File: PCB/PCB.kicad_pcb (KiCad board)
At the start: 2 copper layers, 53.3 x 73.7 mm, 23 parts, among them J1 PWR,A0, J10 D8-D10, J11 D0-D7, J12 GrowLight Out, J2 12V, J3 LightSensor, J4 Pump1, J5 Sensor1, J6 GrowLight In, J7 Pump2, J8 Sensor2, J9 Setup, K1 Relay1, K2 RelayGrowlight, K3 Relay2, Q1 BC337, Q2 BC337, Q3 BC337, U1 AM2302, U2 74HC4051

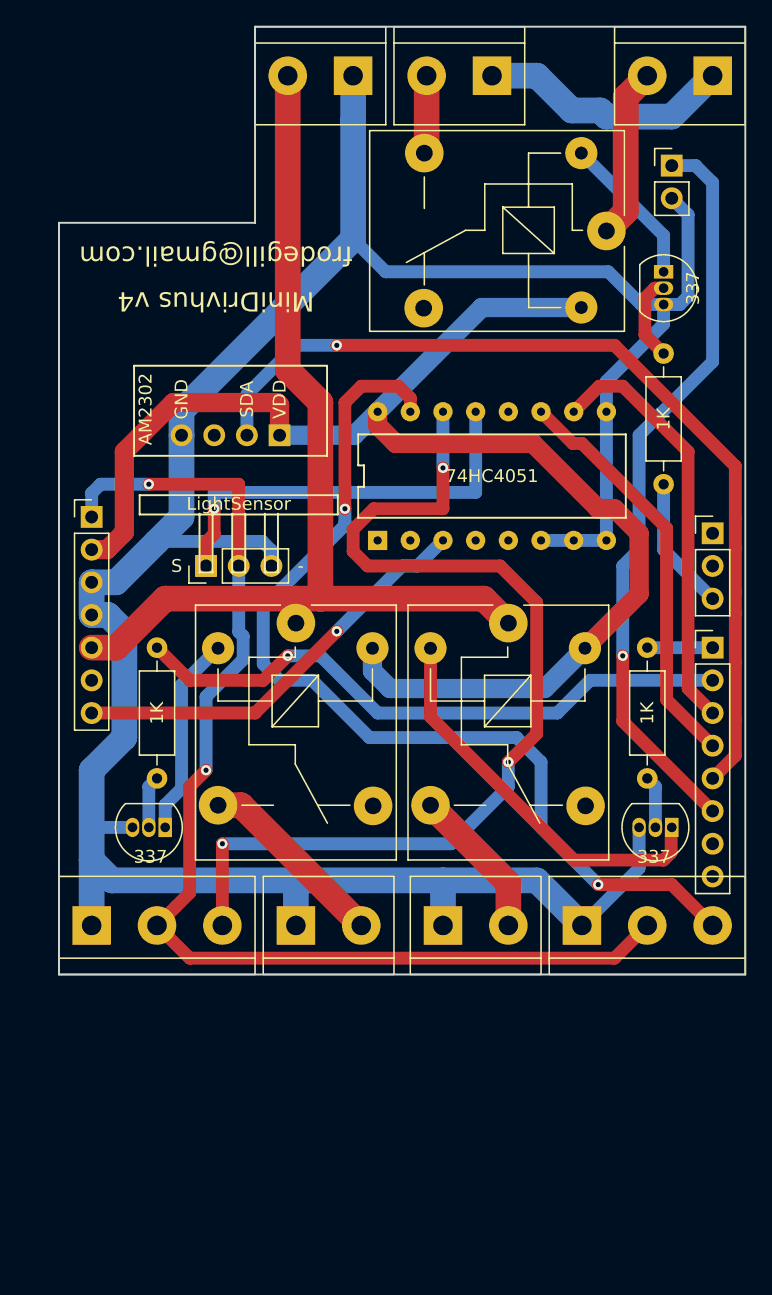
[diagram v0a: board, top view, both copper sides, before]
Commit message: Kicad-files for MivinDrivhus_v5
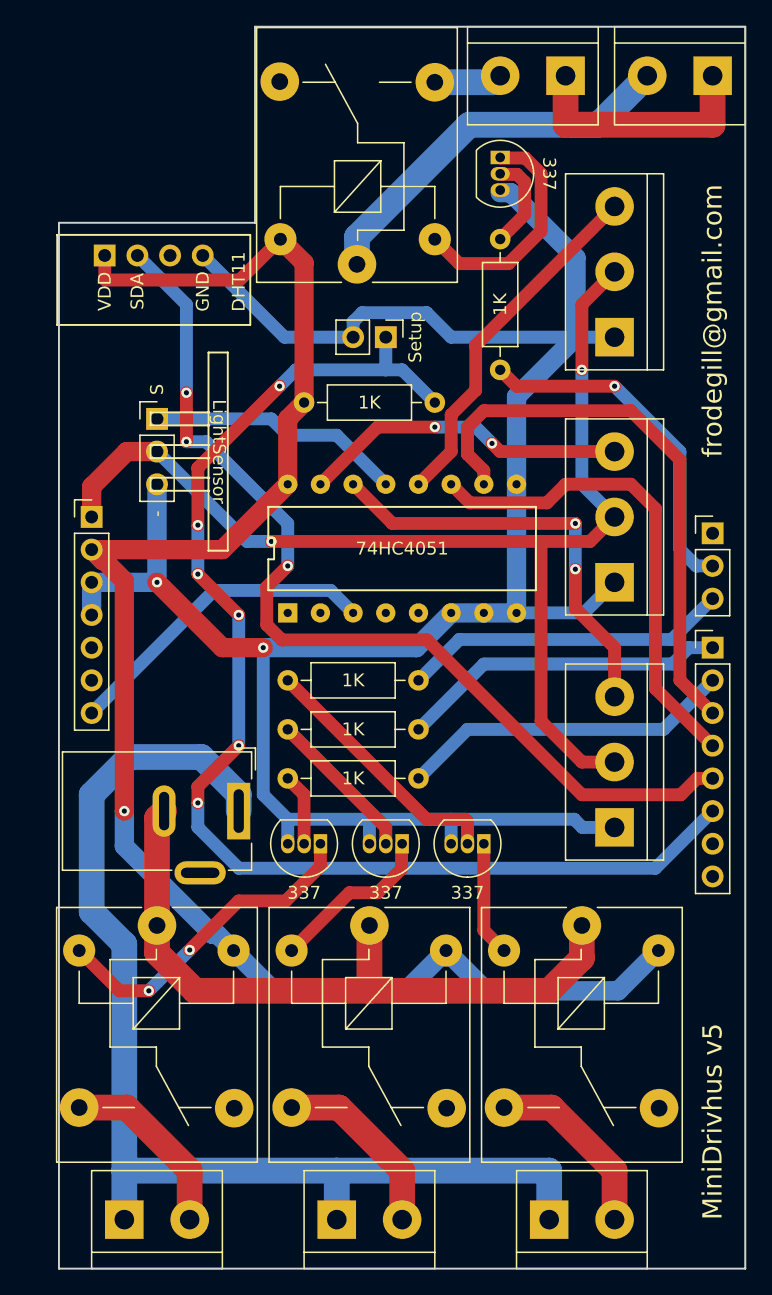
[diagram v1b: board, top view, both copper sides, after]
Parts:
- added J13: Pump3, TerminalBlock:TerminalBlock_bornier-2_P5.08mm, F.Cu at (177.8, 128.3)
- added J14: Sensor3, TerminalBlock:TerminalBlock_bornier-3_P5.08mm, F.Cu at (182.9, 59.7)
- added K4: Relay3, Relay_THT:Relay_SPDT_SANYOU_SRD_Series_Form_C, F.Cu at (180.3, 105.4)
- added Q4: BC337, Package_TO_SOT_THT:TO-92_Inline, F.Cu at (172.7, 99.1)
- added R4: 1K, Resistor_THT:R_Axial_DIN0207_L6.3mm_D2.5mm_P10.16mm_Horizontal, F.Cu at (158.8, 64.8)
- added R5: 1K, Resistor_THT:R_Axial_DIN0207_L6.3mm_D2.5mm_P10.16mm_Horizontal, F.Cu at (157.5, 86.4)
- J2: value 12V -> Pump In; footprint TerminalBlock:TerminalBlock_bornier-2_P5.08mm -> Connector_BarrelJack:BarrelJack_Wuerth_6941xx301002
- U1: value AM2302 -> DHT11
- moved J2 57.8 mm to (153.7, 96.5), turned to 270 degrees
- moved J5 41.3 mm to (182.9, 97.8), turned to 90 degrees
- moved R3 28.2 mm to (157.5, 90.2), turned to 0 degrees
- moved J8 26.8 mm to (182.9, 78.7), turned to 90 degrees
- moved J4 26.5 mm to (144.8, 128.3)
- moved J9 25.9 mm to (165.1, 59.7), turned to 270 degrees
- moved K1 25.9 mm to (147.3, 105.4)
- moved K3 25.9 mm to (163.8, 105.4)
- moved J7 24.3 mm to (161.3, 128.3)
- moved Q3 21.0 mm to (166.4, 99.1)
- moved K2 19.6 mm to (162.9, 54.0), turned to 90 degrees
- moved Q2 15.5 mm to (174.0, 45.7)
- moved R2 15.5 mm to (174.0, 52.1)
- moved U1 15.2 mm to (147.1, 53.3), turned to 0 degrees
- moved Q1 12.1 mm to (160.0, 99.1)
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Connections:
- J1 pad 5: +12V -> (no net)
- J10 pad 2: (no net) -> Net-(J10-Pad2)
- J2 pad 1: GND -> Net-(J13-Pad1)
- J2 pad 2: +12V -> Net-(J2-Pad2)
- J4 pad 1: GND -> Net-(J13-Pad1)
- J7 pad 1: GND -> Net-(J13-Pad1)
- K1 pad 1: +12V -> Net-(J2-Pad2)
- K3 pad 1: +12V -> Net-(J2-Pad2)
- R2 pad 2: Net-(J10-Pad3) -> Net-(J10-Pad2)
- U2 pad 12: (no net) -> Net-(J14-Pad3)
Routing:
- net Net-(J13-Pad1): track 0.00 -> 89.9 mm
- net +12V: track 78.3 -> 0.00 mm
- net Net-(J2-Pad2): track 0.00 -> 54.2 mm
- net Net-(J8-Pad3): track 76.3 -> 25.5 mm
- net Net-(J5-Pad3): track 78.4 -> 33.3 mm, vias 3 -> 2
- net Net-(J11-Pad6): track 58.4 -> 98.9 mm, vias 1 -> 6
- net GND: track 210.4 -> 174.9 mm, vias 0 -> 2
- net Net-(J14-Pad3): track 0.00 -> 27.9 mm
- net Net-(J10-Pad2): track 0.00 -> 27.3 mm, vias 0 -> 1
- net Net-(J11-Pad2): track 47.9 -> 26.0 mm, vias 1 -> 0
- net Net-(J11-Pad1): track 5.08 -> 25.5 mm
- net Net-(Q4-Pad2): track 0.00 -> 20.3 mm
- net +5V: track 108.7 -> 128.7 mm, vias 0 -> 1
- net Net-(K3-Pad2): track 30.9 -> 13.1 mm
- net Net-(J12-Pad2): track 13.4 -> 29.9 mm
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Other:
- board size 53.3 x 73.7 mm -> 53.3 x 96.5 mm
- board text added: "- +"
- board text added: "MiniDrivhus v5"
- board text added: "Pump3"
- board text added: "Sensor3"
- board text removed: "12V"
- board text removed: "3V 5V GND GND 12V A0"
- board text removed: "D10 D9 D8"
- board text removed: "D7 D6 D5 D4 D3 D2 D1 D0"
- board text removed: "GrowLight Relay"
- board text removed: "MiniDrivhus v4"
- board text removed: "Plant 1 Relay"
- board text removed: "Plant 2 Relay"
